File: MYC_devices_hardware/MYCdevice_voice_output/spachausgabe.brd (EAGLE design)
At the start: 86.3 x 56.2 mm, 48 parts, among them IC1 MEGA8-P, IC2 MAX232, IC3 7805TV, Q1 20MHz, X1 8-15V, X2 1503_09, X3 1503_09, X4 RS232, X5 1503_09

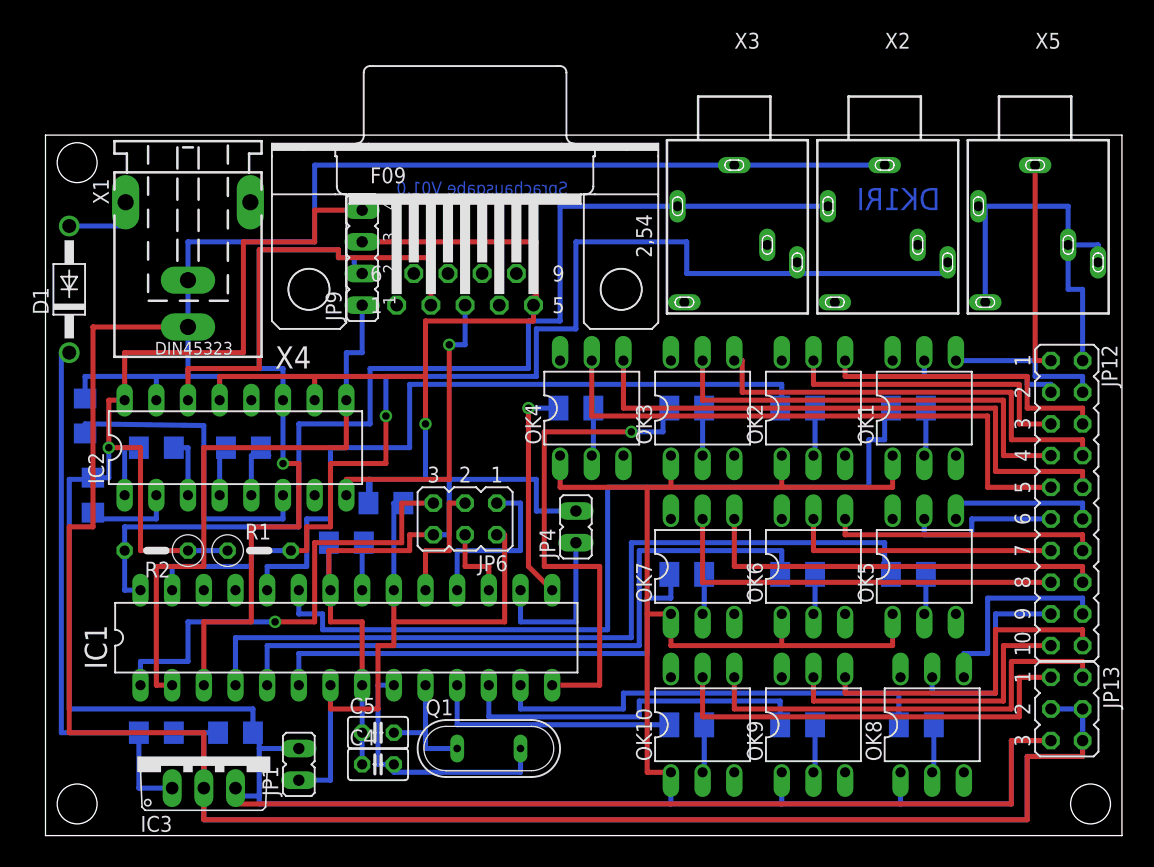
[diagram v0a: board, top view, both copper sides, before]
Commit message: new board (MSM4); bascom with include files
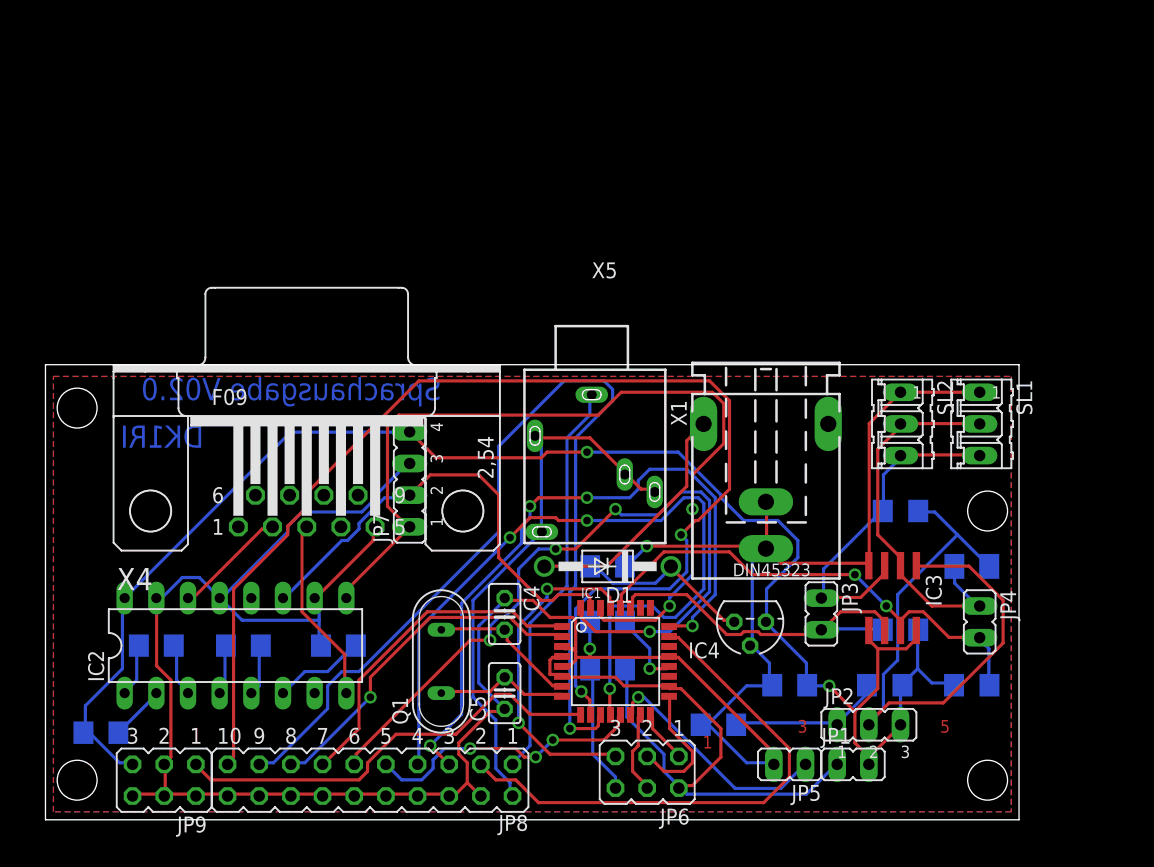
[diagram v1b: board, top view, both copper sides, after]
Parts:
- removed JP12: Modul1, jumper:JP10Q
- removed JP13: Modul2, jumper:JP3Q
- removed OK1, OK10, OK2, OK3, OK4, OK5, OK6, OK7, OK8, OK9: CNY17, optocoupler:DIL06
- removed R10, R11, R12, R7, R8, R9: 1k, resistor:M1206
- removed X2, X3: 1503_09, con-lumberg:1503_09
- added IC4: 78L05Z, linear:TO92
- added JP2: 3V/5V, jumper:JP2
- added JP3: SDA, jumper:JP1
- added JP5: Reset, jumper:JP1
- added JP7: US7, jumper:JP4
- added JP8: Modul1, jumper:JP10Q
- added SL1, SL2: (no value), con-amp-quick:03P
- C1, C2, C3, C6: value 22uF 1210 -> 22uF
- C10, C7, C8, C9: value 22u 1210 -> 22uF
- IC1: value MEGA8-P -> MEGA8-AI; device atmel:DIL28-3 -> atmel:TQFP32-08
- IC3: value 7805TV -> PCA9517; device linear:TO220V -> PCA9517:SO-08
- JP4: value Reset -> SCL
- JP9: value USB -> Modul2; device jumper:JP4 -> jumper:JP3Q
- R1: value 4k7 -> see manual; device resistor:0207/5V -> resistor:R1206
- R2: value 4k7 -> see manual; device resistor:0207/5V -> resistor:M1206
- R3, R4: value 1k -> see manual; device resistor:M1206 -> resistor:R1206
- R5: device resistor:M1206 -> resistor:R1206
- R6: value 1k -> 1k5; device resistor:M1206 -> resistor:R1206
- moved R2 65.4 mm to (74.3, 20.3), flipped to the bottom, turned to 0 degrees
- moved IC3 56.7 mm to (67.9, 17.8), turned to 180 degrees
- moved R1 51.5 mm to (68.6, 24.8), flipped to the bottom
- moved X1 49.6 mm to (57.8, 31.8)
- moved D1 48.6 mm to (45.1, 20.3), turned to 180 degrees
- moved C10 46.6 mm to (45.1, 12.1), turned to 0 degrees
- moved JP9 44.8 mm to (9.53, 3.17), turned to 180 degrees
- moved C2 44.6 mm to (59.7, 10.8)
- moved JP1 44.4 mm to (64.8, 4.45), turned to 270 degrees
- moved X5 40.0 mm to (43.8, 36.2)
- moved C1 38.6 mm to (45.1, 20.3)
- moved JP4 33.3 mm to (74.9, 15.9), turned to 180 degrees
- moved R6 27.9 mm to (54.0, 7.62)
- moved R5 27.3 mm to (67.3, 10.8)
- moved R4 26.3 mm to (74.3, 10.8)
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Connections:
- removed net N$24: JP12.18, OK8.4
- removed net N$31: JP12.17, OK8.5
- removed net N$32: JP12.9, OK4.5
- removed net N$35: C3.2, IC1.21
- removed net N$36: JP12.5, OK2.5
- removed net N$38: JP13.1, OK10.5
- removed net N$40: JP12.19, OK9.5
- removed net N$41: JP12.6, OK2.4
- removed net N$42: JP12.15, OK7.5
- removed net N$43: JP12.7, OK3.5
- removed net N$45: JP12.8, OK3.4
- removed net N$46: JP12.10, OK4.4
- removed net N$47: JP12.11, OK5.5
- removed net N$48: JP12.12, OK5.4
- removed net N$49: OK9.2, R11.2
- removed net N$50: OK8.2, R10.2
- removed net N$53: JP12.13, OK6.5
- removed net N$54: JP12.14, OK6.4
- removed net N$55: JP12.3, OK1.5
- removed net N$56: JP12.4, OK1.4
- removed net N$57: OK7.2, R9.2
- removed net N$58: OK6.2, R8.2
- removed net N$59: OK5.2, R7.2
- removed net N$62: OK4.2, R6.2
- removed net N$64: OK2.2, R4.2
- removed net N$65: OK1.2, R3.2
- net C13: now also C6.1; no longer C7.1
- net GND: now also C10.2, C9.1, IC1.21, IC1.3, IC1.5, IC3.4, IC4.2, JP5.2, JP7.3, JP8.10, JP8.12, JP8.14, JP8.16, JP8.18, JP8.20, JP8.4, JP8.6, JP8.8, JP9.2, JP9.4, JP9.6, R6.1, SL1.1, SL2.1; no longer C10.1, C6.2, IC1.22, IC1.8, IC3.2, JP13.3, JP13.4, JP13.6, JP4.2, X2.1, X3.1
- net N$1: now also IC1.10, JP8.19; no longer IC1.12, R11.1
- net N$10: now also IC3.2, JP4.1, R2.2, SL1.2, SL2.2; no longer OK3.2, R5.2
- net N$11: now also IC3.1, JP2.2, R1.1, R2.1; no longer OK10.2, R12.2
- net N$12: now also IC1.31, JP7.2; no longer IC1.3, JP9.2
- net N$13: now also C7.1; no longer C8.1
- net N$14: now also C6.2; no longer C7.2
- net N$15: now also IC1.16; no longer IC1.18
- net N$16: now also C8.1; no longer C9.1
- net N$17: now also C9.2; no longer C10.2
- net N$18: now also IC1.29; no longer IC1.1
- net N$19: now also IC1.7; no longer IC1.9
- net N$2: now also IC1.30, JP7.1; no longer IC1.2, JP9.1
- net N$20: now also IC1.17; no longer IC1.19
- net N$21: now also JP2.1, R5.1, R6.2; no longer JP12.20, OK9.4
- net N$22: now also IC3.7, JP4.2, R4.2; no longer R2.2, X2.2, X3.2
- net N$23: now also IC1.2, JP8.15; no longer IC1.6, R9.1
- net N$25: now also JP8.5; no longer R4.1
- net N$26: now also IC1.12, JP8.7; no longer IC1.14, R5.1
- net N$28: now also IC1.15; no longer IC1.17
- net N$29: now also C3.2, IC1.20; no longer JP12.16, OK7.4
- net N$3: now also C7.2; no longer C8.2
- net N$30: now also IC1.9, JP9.1; no longer IC1.11, R12.1
- net N$33: now also IC4.3; no longer IC3.1
- net N$34: now also JP8.3; no longer R3.1
- net N$37: now also IC1.8; no longer IC1.10
- net N$39: now also IC1.13, JP8.9; no longer IC1.15, R6.1
- net N$44: now also C10.1, IC1.18, IC1.4, IC1.6; no longer C6.1, IC1.20, IC1.7
- net N$5: now also IC3.6, JP3.2, R3.2; no longer R1.2, X2.3, X3.3
- net N$51: now also IC1.1, JP8.13; no longer IC1.5, R8.1
- net N$52: now also IC1.32, JP8.11; no longer IC1.4, R7.1
- net N$6: now also IC1.14, JP5.1; no longer IC1.16, JP4.1
- net N$60: now also JP8.1; no longer JP12.1
- net N$61: now also JP8.2; no longer JP12.2
- net N$7: now also IC1.11, JP8.17; no longer IC1.13, R10.1
- net N$8: now also IC3.3, JP3.1, R1.2, SL1.3, SL2.3; no longer JP13.2, OK10.4
- net VDD: now also C8.2, IC3.5, IC3.8, IC4.1, JP2.3, JP7.4, JP9.5, R3.1, R4.1, R5.2; no longer C9.2, IC3.3, JP13.5, JP9.4, OK1.1, OK10.1, OK2.1, OK3.1, OK4.1, OK5.1, OK6.1, OK7.1, OK8.1, OK9.1, R1.1, R2.1
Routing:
- net GND: track 447.9 -> 232.7 mm, vias 1 -> 2
- net VDD: track 346.6 -> 131.8 mm, vias 1 -> 2
- net N$1: track 29.2 -> 97.5 mm, vias 0 -> 2
- net N$5: track 94.5 -> 29.5 mm, vias 1 -> 0
- net N$22: track 88.5 -> 39.7 mm, vias 0 -> 2
- net N$46: track 47.0 -> 0.00 mm
- net N$32: track 47.0 -> 0.00 mm
- net N$11: track 3.94 -> 50.8 mm
- net N$7: track 36.8 -> 78.5 mm, vias 0 -> 1
- net N$45: track 35.6 -> 0.00 mm
- net N$43: track 35.6 -> 0.00 mm
- net N$38: track 34.3 -> 0.00 mm
- net N$42: track 33.0 -> 0.00 mm
- net N$33: track 44.5 -> 14.6 mm
- net N$10: track 3.82 -> 31.5 mm
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- added copper zone on layer 1, net GND
- added copper zone on layer 16, net GND
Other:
- board size 86.3 x 56.2 mm -> 78.1 x 36.5 mm
- board text added: "1"
- board text added: "3"
- board text added: "5"
- board text added: "Sprachausgabe V02.0"
- board text removed: "Sprachausgabe V01.0"
